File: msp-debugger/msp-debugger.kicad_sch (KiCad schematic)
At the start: 2 parts, among them U1 ESP32-WROOM-32, U2 NHD-0420H1Z

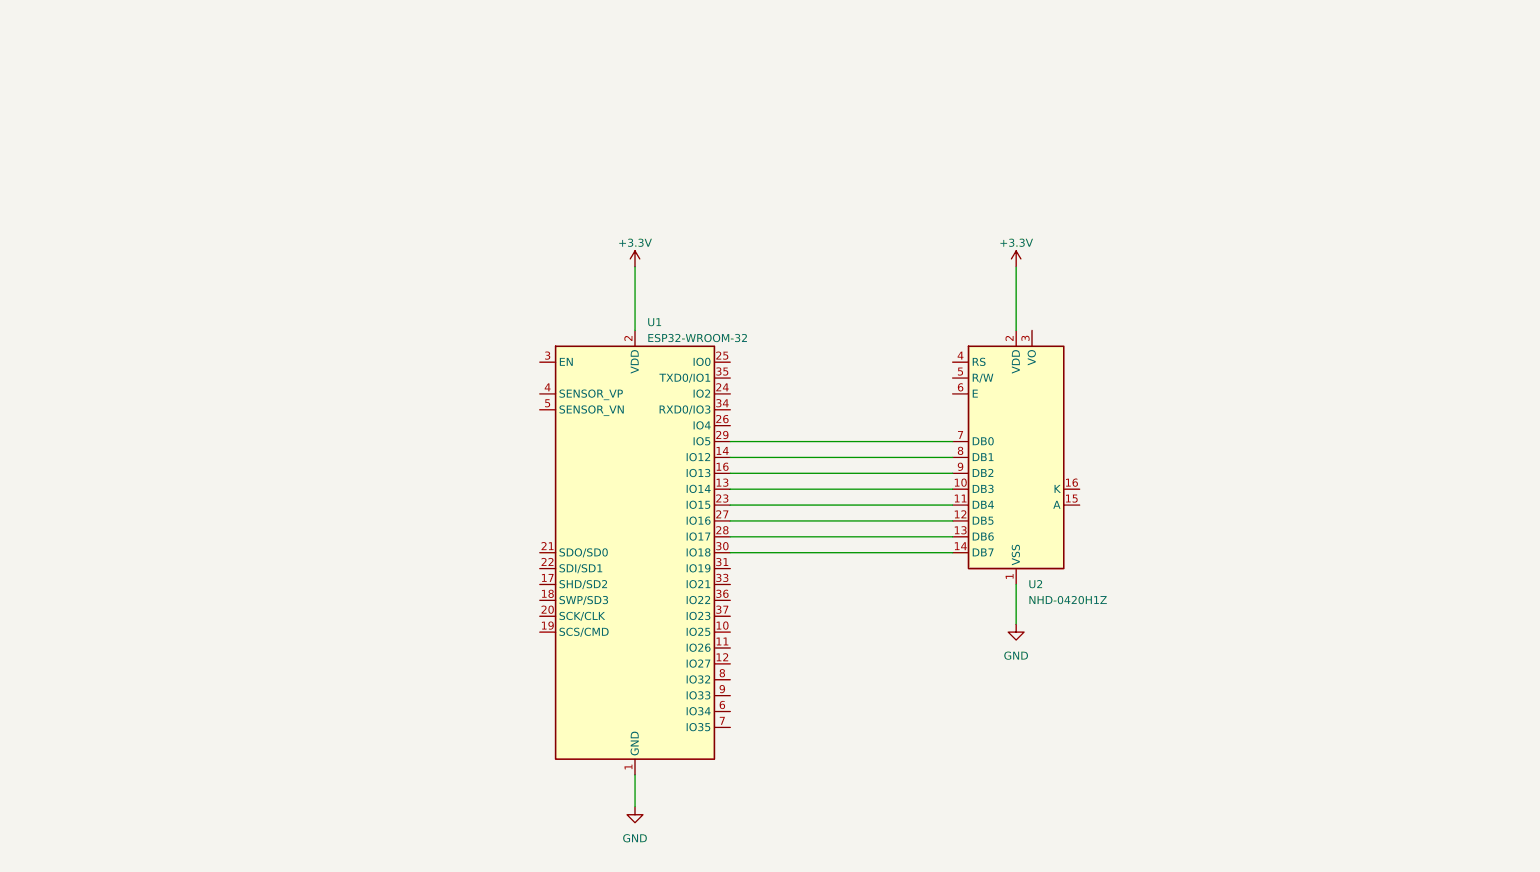
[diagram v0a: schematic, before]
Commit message: working on things
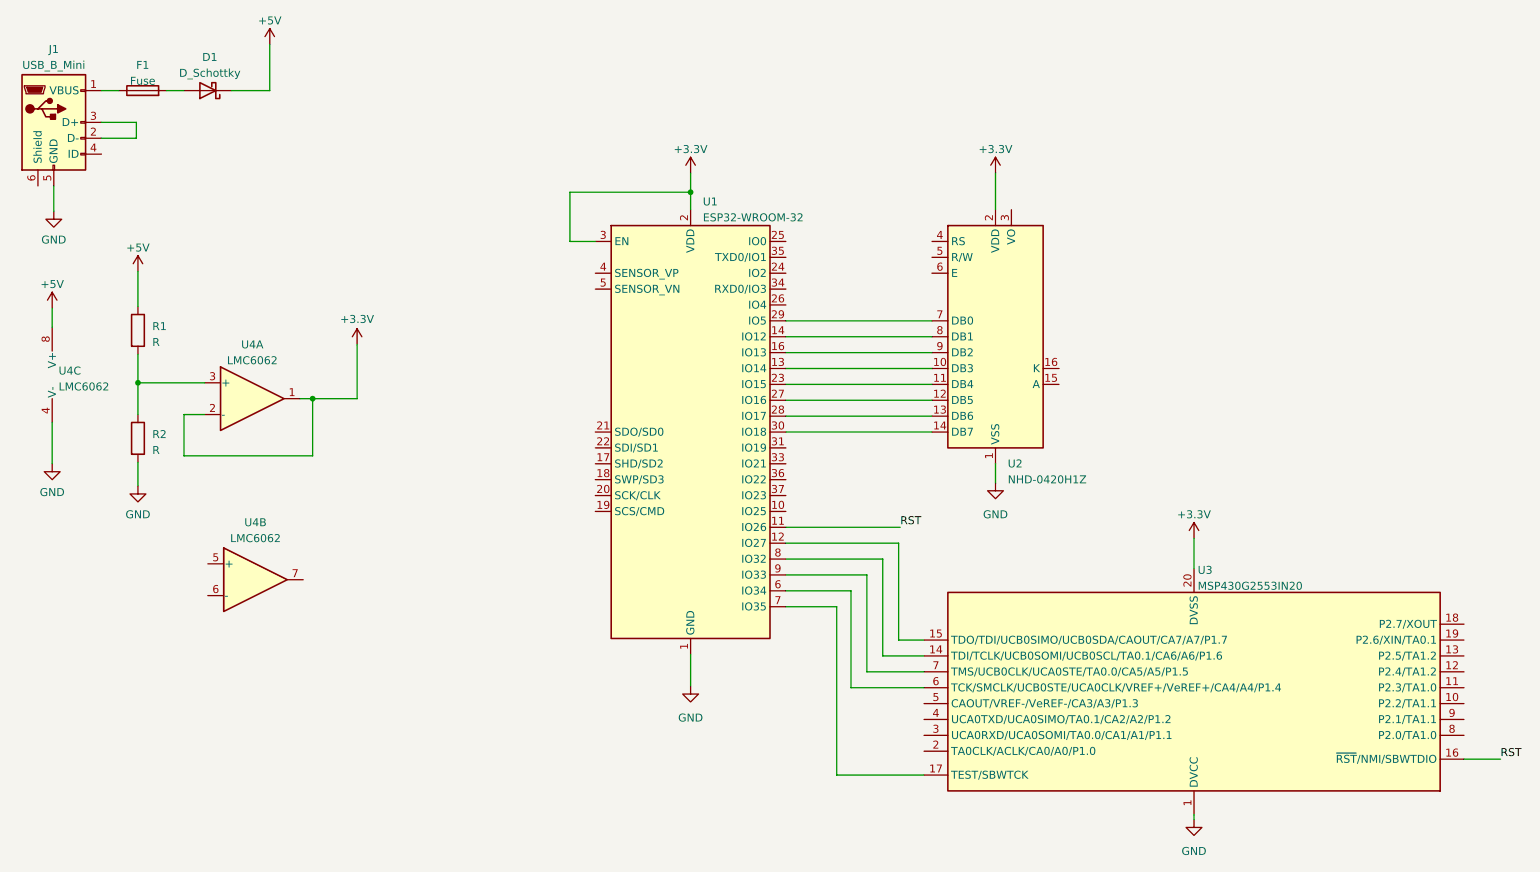
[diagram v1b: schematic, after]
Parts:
- added D1: D_Schottky, symbol Device:D_Schottky
- added F1: Fuse, symbol Device:Fuse
- added J1: USB_B_Mini, symbol Connector:USB_B_Mini
- added R1, R2: R, symbol Device:R
- added U3: MSP430G2553IN20, Package_DIP:DIP-20_W7.62mm, symbol MCU_Texas_MSP430:MSP430G2553IN20
- added U4: LMC6062, symbol Amplifier_Operational:LMC6062
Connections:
- net +3.3V: now also U1.3 (EN), U3.20 (DVSS), U4.1, U4.2 (-)
- net GND: now also J1.5 (GND), R2.2, U3.1 (DVCC), U4.4 (V-)
- net RST: now reaches U1.11 (IO26)
- net RST: now also U3.16 (~{RST}/NMI/SBWTDIO)
- net at U1.12 (IO27): now also U3.15 (TDO/TDI/UCB0SIMO/UCB0SDA/CAOUT/CA7/A7/P1.7)
- net at U1.6 (IO34): now also U3.6 (TCK/SMCLK/UCB0STE/UCA0CLK/VREF+/VeREF+/CA4/A4/P1.4)
- net at U1.7 (IO35): now also U3.17 (TEST/SBWTCK)
- net at U1.8 (IO32): now also U3.14 (TDI/TCLK/UCB0SOMI/UCB0SCL/TA0.1/CA6/A6/P1.6)
- net at U1.9 (IO33): now also U3.7 (TMS/UCB0CLK/UCA0STE/TA0.0/CA5/A5/P1.5)
- new net: R1.2, R2.1, U4.3 (+)
- new net: D1.2 (A), F1.2
- new net: F1.1, J1.1 (VBUS)
- new net: J1.2 (D-), J1.3 (D+)
- new net +5V: D1.1 (K), R1.1, U4.8 (V+)
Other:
- moved on the sheet: U1, U2
